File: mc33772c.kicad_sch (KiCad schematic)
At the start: 11 parts, among them U2 MC33772CTP1AE

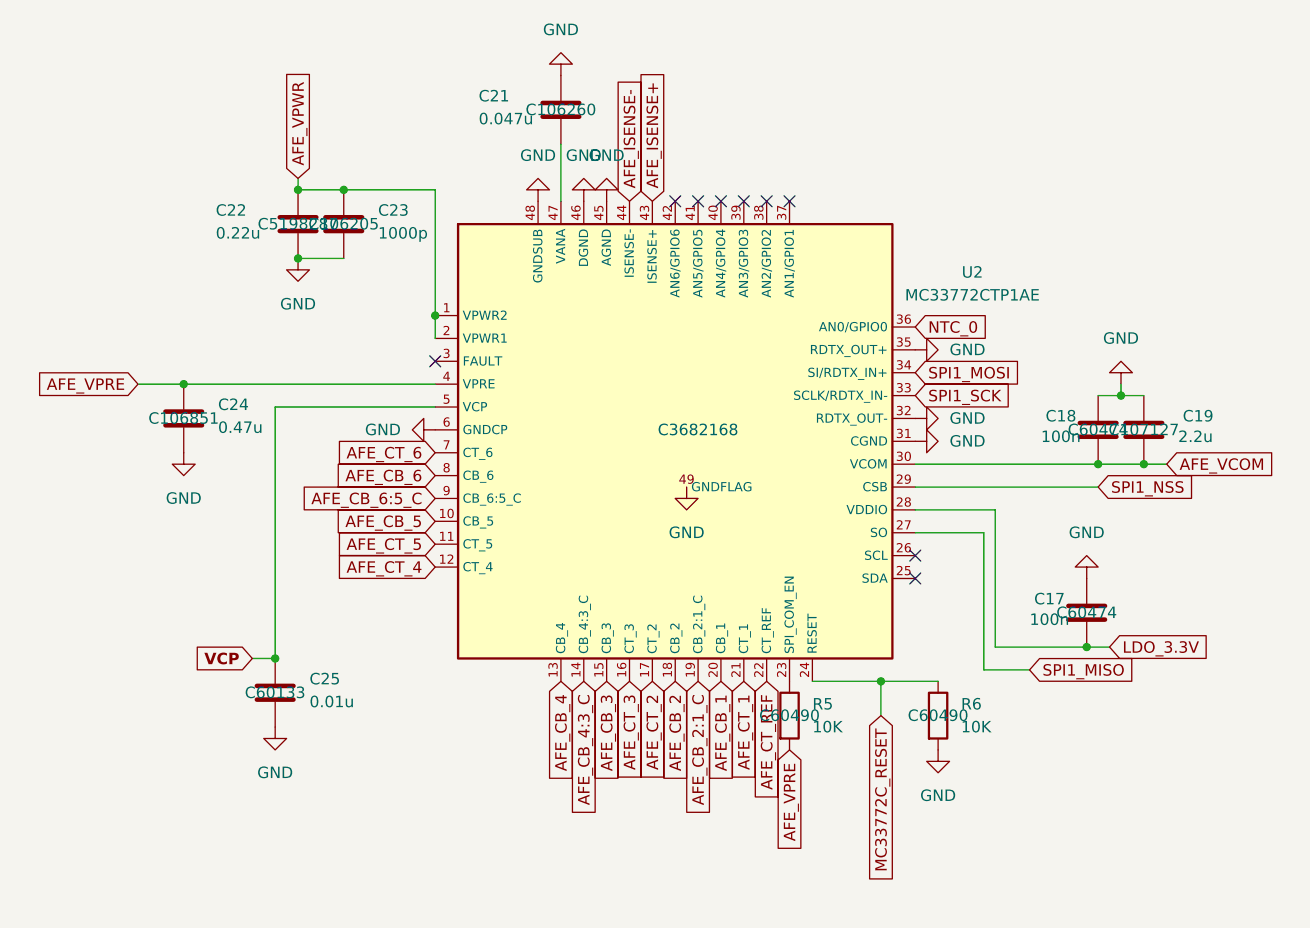
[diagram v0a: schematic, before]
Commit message: for PCBWay
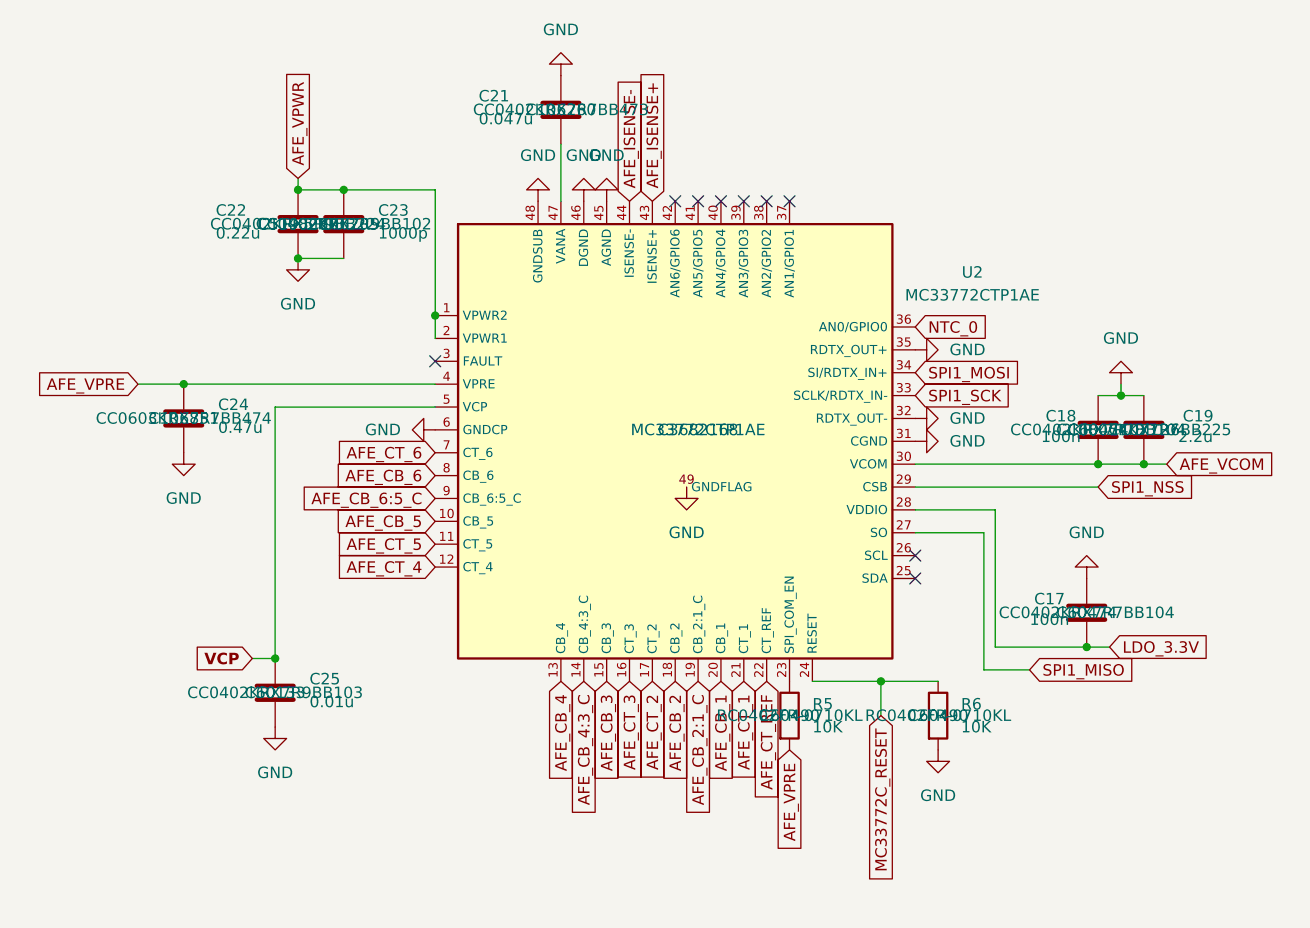
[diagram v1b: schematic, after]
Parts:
- C17, C18: MPN (none) -> CC0402KRX7R7BB104
- C19: MPN (none) -> CC0805KKX7R6BB225
- C21: MPN (none) -> CC0402KRX7R7BB473
- C22: MPN (none) -> CC0402KRX5R9BB224
- C23: MPN (none) -> CC0402KRX7R9BB102
- C24: MPN (none) -> CC0603KRX7R7BB474
- C25: MPN (none) -> CC0402KRX7R9BB103
- R5, R6: MPN (none) -> RC0402FR-0710KL
- U2: MPN (none) -> MC33772CTP1AE
